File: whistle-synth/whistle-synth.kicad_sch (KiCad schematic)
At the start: 14 parts

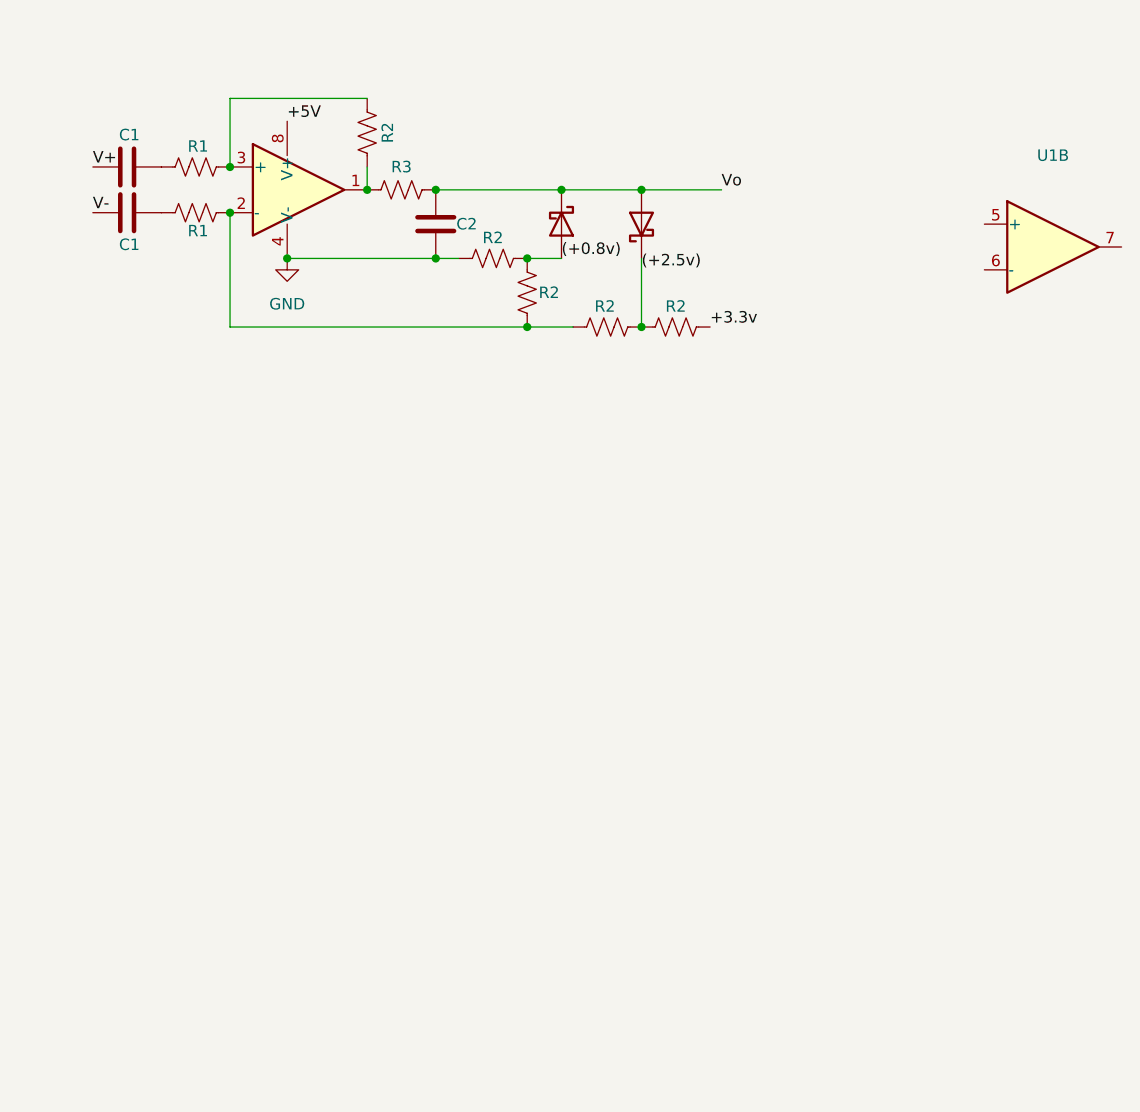
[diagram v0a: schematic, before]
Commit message: whistle synth pre-amp v1
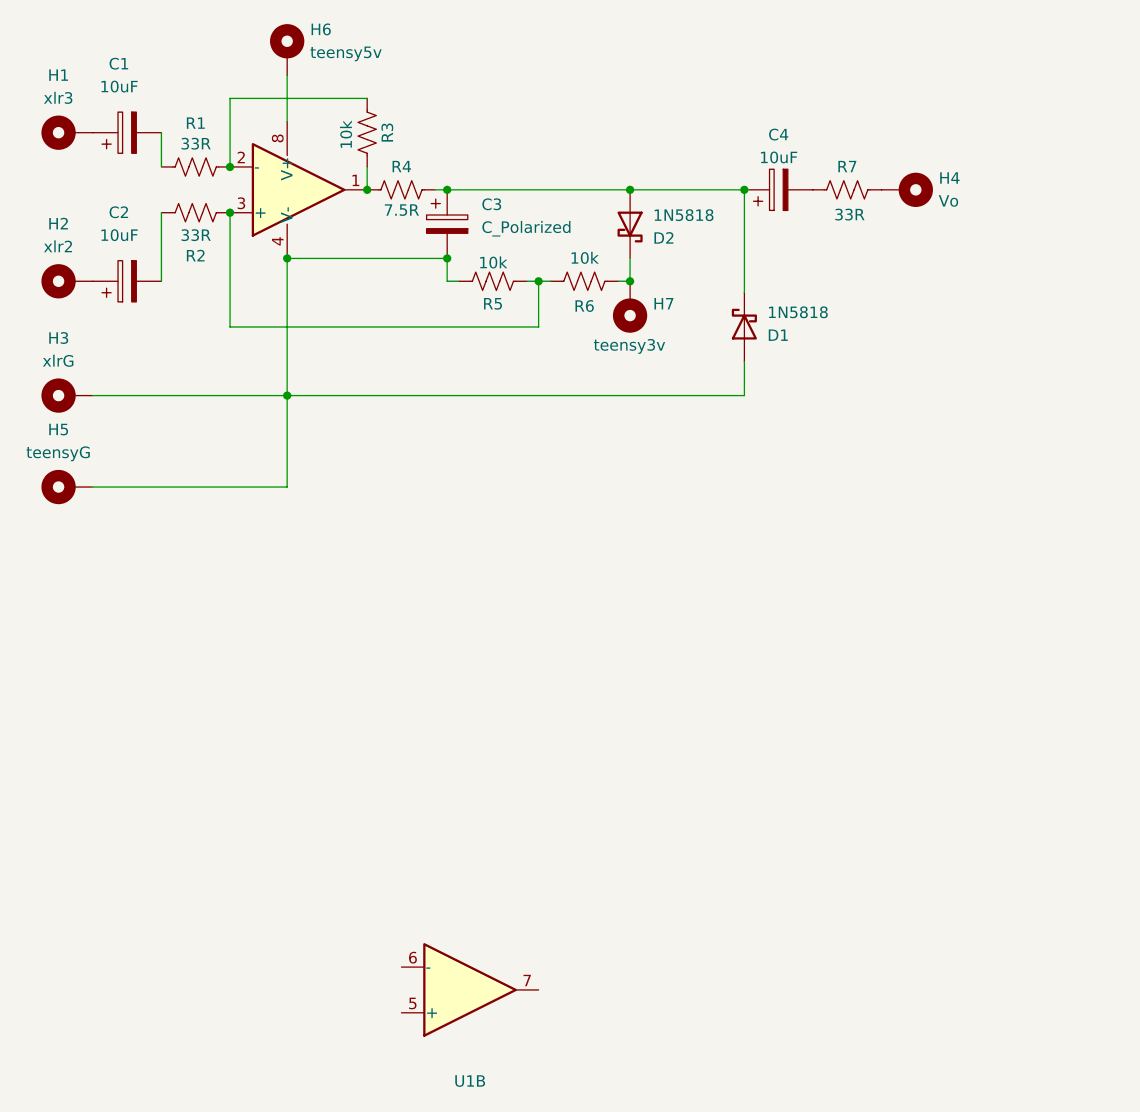
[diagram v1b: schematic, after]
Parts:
- removed C1 (x2), C2: ~, symbol Device:C
- removed D1 (x2): ~, Diode_THT:D_DO-41_SOD81_P10.16mm_Horizontal, symbol Diode:1N5817
- removed R2 (x2): ~, symbol Device:R_US
- added C1, C2, C4: 10uF, Capacitor_THT:CP_Radial_D4.0mm_P2.00mm, symbol Device:C_Polarized
- added C3: C_Polarized, Capacitor_THT:CP_Radial_D4.0mm_P2.00mm, symbol Device:C_Polarized
- added D1, D2: 1N5818, Diode_THT:D_DO-41_SOD81_P10.16mm_Horizontal, symbol Diode:1N5818
- added H1: xlr3, MountingHole:MountingHole_2.2mm_M2_DIN965_Pad_TopBottom, symbol Mechanical:MountingHole_Pad
- added H2: xlr2, MountingHole:MountingHole_2.2mm_M2_DIN965_Pad_TopBottom, symbol Mechanical:MountingHole_Pad
- added H3: xlrG, MountingHole:MountingHole_2.2mm_M2_DIN965_Pad_TopBottom, symbol Mechanical:MountingHole_Pad
- added H4: Vo, MountingHole:MountingHole_2.2mm_M2_DIN965_Pad_TopBottom, symbol Mechanical:MountingHole_Pad
- added H5: teensyG, MountingHole:MountingHole_2.2mm_M2_DIN965_Pad_TopBottom, symbol Mechanical:MountingHole_Pad
- added H6: teensy5v, MountingHole:MountingHole_2.2mm_M2_DIN965_Pad_TopBottom, symbol Mechanical:MountingHole_Pad
- added H7: teensy3v, MountingHole:MountingHole_2.2mm_M2_DIN965_Pad_TopBottom, symbol Mechanical:MountingHole_Pad
- added R7: 33R, Resistor_THT:R_Axial_DIN0309_L9.0mm_D3.2mm_P12.70mm_Horizontal, symbol Device:R_US
- R1: value ~ -> 33R; footprint (none) -> Resistor_THT:R_Axial_DIN0309_L9.0mm_D3.2mm_P12.70mm_Horizontal
- R2: renamed from R1; value ~ -> 33R; footprint (none) -> Resistor_THT:R_Axial_DIN0309_L9.0mm_D3.2mm_P12.70mm_Horizontal
- R3, R5, R6: renamed from R2; value ~ -> 10k; footprint (none) -> Resistor_THT:R_Axial_DIN0309_L9.0mm_D3.2mm_P12.70mm_Horizontal
- R4: renamed from R3; value ~ -> 7.5R; footprint (none) -> Resistor_THT:R_Axial_DIN0309_L9.0mm_D3.2mm_P12.70mm_Horizontal
- U1: footprint (none) -> Package_DIP:DIP-8_W7.62mm
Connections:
- net (+0.8v) is gone; now on an unnamed net: R5.1
- net (+2.5v) is gone; now on an unnamed net: R6.2
- net at R1.1, R3.2: now also U1.2 (-); no longer U1.3 (+)
- net at R1.2: now also C1.2
- net at R2.2: now also C2.2
- net at R2.1: now also U1.3 (+); no longer U1.2 (-)
- net +3.3v: no longer names the net of R6.1
- net +3.3v: now also D2.1 (K), H7.1
- net +5V: no longer names the net of U1.8 (V+)
- net +5V: now also H6.1
- net GND: no longer names the net of R5.2, U1.4 (V-)
- net GND: now also C3.2, D1.2 (A), H3.1, H5.1
- net Vo: no longer names the net of R4.1
- net Vo: now also C3.1, C4.1, D1.1 (K), D2.2 (A)
- new net: C1.1, H1.1
- new net: C4.2, R7.2
- new net: C2.1, H2.1
- new net: H4.1, R7.1
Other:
- moved on the sheet: R5, R6, U1B
